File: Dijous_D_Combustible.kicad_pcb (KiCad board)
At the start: 2 copper layers, 90 x 75 mm, 64 parts, among them J1 Screw_Terminal_01x02, J2 Conn_01x02, J3 Conn_02x03_Counter_Clockwise, J4 DE9_Plug, J5 Conn_01x02, J6 Conn_01x02, J7 Conn_01x02, K1 Fujitsu_FTR-LYAA005x, K2 Fujitsu_FTR-LYAA005x, Q1 2SC4213, Q2 2SC4213, SW1 SW_Push, U1 MCP2551-I-SN, U2 LM2596S-ADJ, U3 PIC18F258-I/SO, U4 LM1117DT-5.0, U5 MCP4725xxx-xCH, Y1 HC-49-US

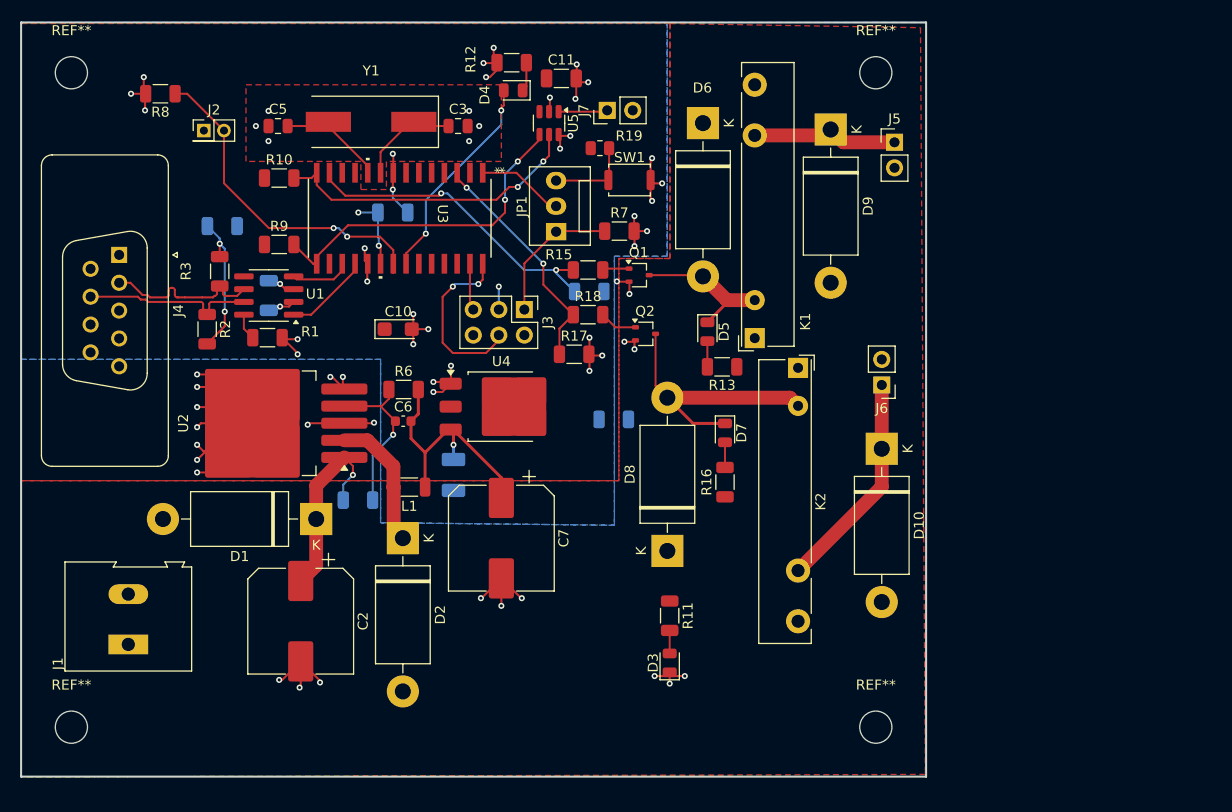
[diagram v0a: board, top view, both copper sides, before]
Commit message: Layout & README
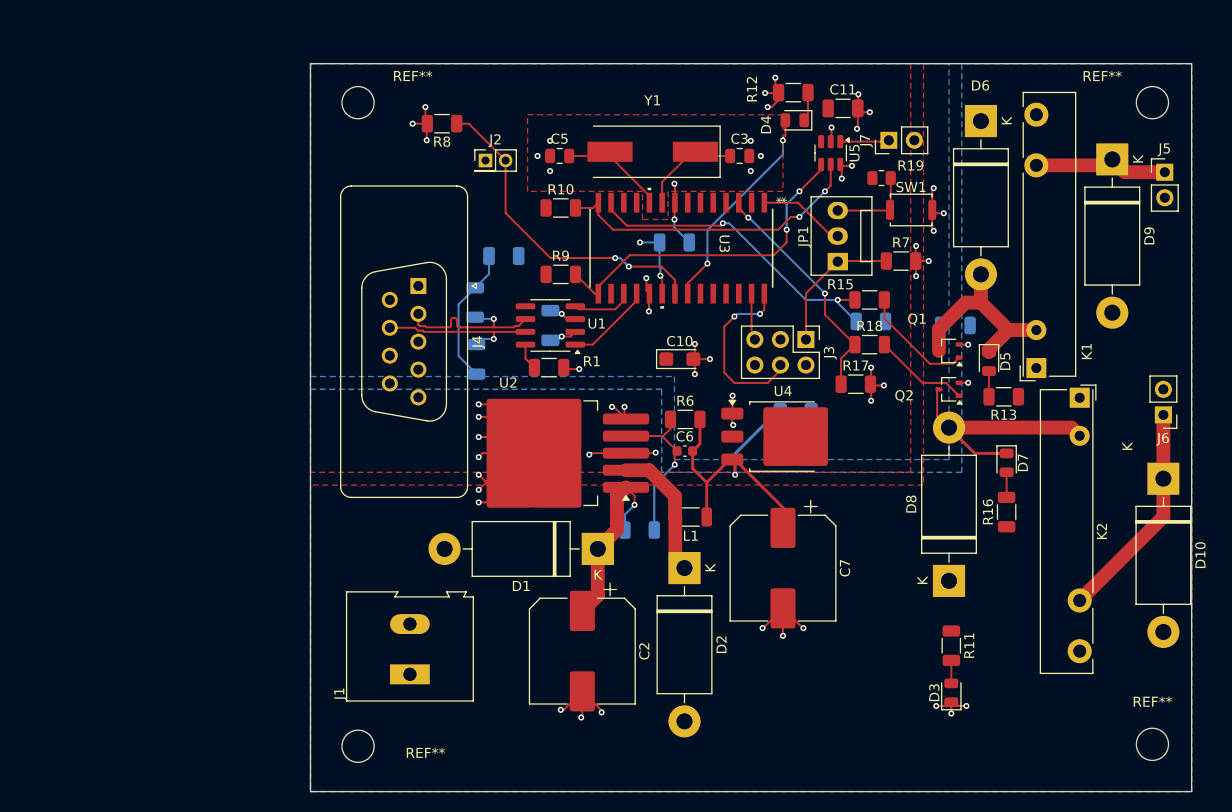
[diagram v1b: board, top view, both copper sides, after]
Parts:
- removed the REF** at (184.5, 137.1)
- removed the REF** at (104.5, 137.1)
- removed the REF** at (104.5, 72.0)
- removed the REF** at (184.5, 72.0)
- added REF**: MountingHole_3.2mm_M3, MountingHole:MountingHole_3.2mm_M3, F.Cu at (133.0, 75.0)
- added REF**: MountingHole_3.2mm_M3, MountingHole:MountingHole_3.2mm_M3, F.Cu at (133.0, 139.0)
- added REF**: MountingHole_3.2mm_M3, MountingHole:MountingHole_3.2mm_M3, F.Cu at (212.0, 138.8)
- added REF**: MountingHole_3.2mm_M3, MountingHole:MountingHole_3.2mm_M3, F.Cu at (212.0, 75.0)
- R2, R3: moved to B.Cu
- moved R4 35.2 mm to (192.4, 97.2)
- moved C8 34.6 mm to (176.5, 106.0), turned to 0 degrees
- moved Q1 31.7 mm to (191.8, 99.7), turned to 180 degrees
- moved Q2 30.7 mm to (191.8, 103.5), turned to 180 degrees
- moved J4 29.9 mm to (139.0, 93.2)
- moved C10 28.2 mm to (165.0, 100.5)
- moved C11 28.2 mm to (181.2, 75.6)
- moved C3 28.2 mm to (171.0, 80.3)
- moved C5 28.2 mm to (153.1, 80.3)
- moved C6 28.2 mm to (165.5, 109.7)
- moved C9 28.2 mm to (164.5, 88.9)
- moved D3 28.2 mm to (192.0, 133.7)
- moved D4 28.2 mm to (176.4, 76.8)
- moved D5 28.2 mm to (195.8, 100.8)
- moved D7 28.2 mm to (197.5, 110.8)
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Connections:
- C1 pad 1: (no net) -> +5V
- C1 pad 2: (no net) -> GND
- C10 pad 1: (no net) -> +5V
- C10 pad 2: (no net) -> GND
- C11 pad 1: (no net) -> +5V
- C11 pad 2: (no net) -> GND
- C2 pad 1: (no net) -> Vin_Buck
- C2 pad 2: (no net) -> GNDPWR
- C3 pad 1: (no net) -> /OSC1
- C3 pad 2: (no net) -> GND
- C4 pad 1: (no net) -> Net-(C4-Pad1)
- C4 pad 2: (no net) -> GND
- C5 pad 1: (no net) -> GND
- C5 pad 2: (no net) -> /OSC2
- C6 pad 1: (no net) -> Net-(U2-FB)
- C6 pad 2: (no net) -> Vin_LDO
- C7 pad 1: (no net) -> Vin_LDO
- C7 pad 2: (no net) -> GNDPWR
- C8 pad 1: (no net) -> Vin_LDO
- C8 pad 2: (no net) -> GND
- C9 pad 1: (no net) -> GND
- C9 pad 2: (no net) -> +5V
- D1 pad 1: (no net) -> Vin_Buck
- D1 pad 2: (no net) -> Vbat
- D10 pad 1: (no net) -> Solenoide
- D10 pad 2: (no net) -> GNDPWR
- D2 pad 1: (no net) -> Vout_Buck
- D2 pad 2: (no net) -> GNDPWR
- D3 pad 1: (no net) -> GNDPWR
- D3 pad 2: (no net) -> Net-(D3-A)
- D4 pad 1: (no net) -> Net-(D4-K)
- D4 pad 2: (no net) -> LED_pneumatics
- D5 pad 1: (no net) -> Retorn_sol
- D5 pad 2: (no net) -> Net-(D5-A)
- D6 pad 1: (no net) -> Vbat
- D6 pad 2: (no net) -> Retorn_sol
- D7 pad 1: (no net) -> Retorn_dip
- D7 pad 2: (no net) -> Net-(D7-A)
- D8 pad 1: (no net) -> Vbat
- D8 pad 2: (no net) -> Retorn_dip
- D9 pad 1: (no net) -> Bomba_combustible
- D9 pad 2: (no net) -> GNDPWR
- J1 pad 1: (no net) -> GNDPWR
- J1 pad 2: (no net) -> Vbat
- J2 pad 1: (no net) -> GND
- J2 pad 2: (no net) -> Boto
- J3 pad 1: (no net) -> MCLR
- J3 pad 2: (no net) -> +5V
- J3 pad 3: (no net) -> GND
- J3 pad 4: (no net) -> PGD
- J3 pad 5: (no net) -> PGC
- J3 pad 6: (no net) -> unconnected-(J3-Pin_6-Pad6)
- J4 pad 1: (no net) -> unconnected-(J4-Pad1)
- J4 pad 2: (no net) -> /Can-
- J4 pad 3: (no net) -> unconnected-(J4-Pad3)
- J4 pad 4: (no net) -> unconnected-(J4-Pad4)
- J4 pad 5: (no net) -> unconnected-(J4-Pad5)
- J4 pad 6: (no net) -> unconnected-(J4-Pad6)
- J4 pad 7: (no net) -> /Can+
- J4 pad 8: (no net) -> unconnected-(J4-Pad8)
- J4 pad 9: (no net) -> unconnected-(J4-Pad9)
- J5 pad 1: (no net) -> Bomba_combustible
- J5 pad 2: (no net) -> GNDPWR
- J6 pad 1: (no net) -> Solenoide
- J6 pad 2: (no net) -> GNDPWR
- J7 pad 1: (no net) -> Nivell_combustible
- J7 pad 2: (no net) -> GND
- JP1 pad 1: (no net) -> MCLR
- JP1 pad 2: (no net) -> Net-(JP1-C)
- JP1 pad 3: (no net) -> Net-(JP1-B)
- K1 pad 13: (no net) -> Bomba_combustible
- K1 pad 14: (no net) -> Vbat
- K1 pad A1: (no net) -> Vbat
- K1 pad A2: (no net) -> Retorn_sol
- K2 pad 13: (no net) -> Solenoide
- K2 pad 14: (no net) -> Vbat
- K2 pad A1: (no net) -> Vbat
- K2 pad A2: (no net) -> Retorn_dip
- L1 pad 1: (no net) -> Vin_LDO
- L1 pad 2: (no net) -> Vout_Buck
- Q1 pad 1: (no net) -> Net-(Q1-B)
- Q1 pad 2: (no net) -> GNDPWR
- Q1 pad 3: (no net) -> Retorn_sol
- Q2 pad 1: (no net) -> Net-(Q2-B)
- Q2 pad 2: (no net) -> GNDPWR
- Q2 pad 3: (no net) -> Retorn_dip
- R1 pad 1: (no net) -> Net-(U1-Rs)
- R1 pad 2: (no net) -> GND
- R10 pad 1: (no net) -> +5V
- R10 pad 2: (no net) -> SCL
- R11 pad 1: (no net) -> Vbat
- R11 pad 2: (no net) -> Net-(D3-A)
- R12 pad 1: (no net) -> Net-(D4-K)
- R12 pad 2: (no net) -> GND
- R13 pad 1: (no net) -> Vbat
- R13 pad 2: (no net) -> Net-(D5-A)
- R14 pad 1: (no net) -> R_Bomba
- R14 pad 2: (no net) -> GND
- R15 pad 1: (no net) -> R_Bomba
- R15 pad 2: (no net) -> Net-(Q1-B)
- R16 pad 1: (no net) -> Vbat
- R16 pad 2: (no net) -> Net-(D7-A)
- R17 pad 1: (no net) -> R_Dipòsit
- R17 pad 2: (no net) -> GND
- R18 pad 1: (no net) -> R_Dipòsit
- R18 pad 2: (no net) -> Net-(Q2-B)
- R19 pad 1: (no net) -> +5V
- R19 pad 2: (no net) -> Net-(JP1-B)
- R2 pad 1: (no net) -> /Can+
- R2 pad 2: (no net) -> Net-(C4-Pad1)
- R3 pad 1: (no net) -> Net-(C4-Pad1)
- R3 pad 2: (no net) -> /Can-
- R4 pad 1: (no net) -> GNDPWR
- R4 pad 2: (no net) -> GND
- R5 pad 1: (no net) -> Net-(U2-FB)
- R5 pad 2: (no net) -> Vin_Buck
- R6 pad 1: (no net) -> Net-(U2-FB)
- R6 pad 2: (no net) -> Vin_LDO
- R7 pad 1: (no net) -> MCLR
- R7 pad 2: (no net) -> GND
- R8 pad 1: (no net) -> Boto
- R8 pad 2: (no net) -> GND
- R9 pad 1: (no net) -> +5V
- R9 pad 2: (no net) -> SCA
- SW1 pad 1: (no net) -> Net-(JP1-B)
- SW1 pad 2: (no net) -> GND
- U1 pad 1: (no net) -> TXD
- U1 pad 2: (no net) -> GND
- U1 pad 3: (no net) -> +5V
- U1 pad 4: (no net) -> RXD
- U1 pad 5: (no net) -> unconnected-(U1-Vref-Pad5)
- U1 pad 6: (no net) -> /Can-
- U1 pad 7: (no net) -> /Can+
- U1 pad 8: (no net) -> Net-(U1-Rs)
- U2 pad 1: (no net) -> Vin_Buck
- U2 pad 2: (no net) -> Vout_Buck
- U2 pad 3: (no net) -> GNDPWR
- U2 pad 4: (no net) -> Net-(U2-FB)
- U2 pad 5: (no net) -> GNDPWR
- U3 pad 1: (no net) -> Net-(JP1-C)
- U3 pad 10: (no net) -> /OSC2
- U3 pad 11: (no net) -> unconnected-(U3A-RC0/T1OSO/T1CK1-Pad11)
- U3 pad 12: (no net) -> unconnected-(U3A-RC1/T1OSI-Pad12)
- U3 pad 13: (no net) -> R_Bomba
- U3 pad 14: (no net) -> SCL
- U3 pad 15: (no net) -> SCA
- U3 pad 16: (no net) -> unconnected-(U3A-RC5/SDO-Pad16)
- U3 pad 17: (no net) -> RXD
- U3 pad 18: (no net) -> TXD
- U3 pad 19: (no net) -> GND
- U3 pad 2: (no net) -> unconnected-(U3A-RA0/AN0/CVREF-Pad2)
- U3 pad 20: (no net) -> +5V
- U3 pad 21: (no net) -> Boto
- U3 pad 22: (no net) -> LED_pneumatics
- U3 pad 23: (no net) -> unconnected-(U3A-RB2/CANTX/INT2-Pad23)
- U3 pad 24: (no net) -> unconnected-(U3A-RB3/CANRX-Pad24)
- U3 pad 25: (no net) -> unconnected-(U3A-RB4-Pad25)
- U3 pad 26: (no net) -> unconnected-(U3A-RB5/PGM-Pad26)
- U3 pad 27: (no net) -> PGC
- U3 pad 28: (no net) -> PGD
- U3 pad 3: (no net) -> R_Dipòsit
- U3 pad 4: (no net) -> unconnected-(U3A-RA2/AN2/VREF--Pad4)
- U3 pad 5: (no net) -> unconnected-(U3A-RA3/AN3/VREF+-Pad5)
- U3 pad 6: (no net) -> unconnected-(U3A-RA4/T0CKI-Pad6)
- U3 pad 7: (no net) -> unconnected-(U3A-RA5/AN4/*SS/LVDIN-Pad7)
- U3 pad 8: (no net) -> GND
- U3 pad 9: (no net) -> /OSC1
- U4 pad 1: (no net) -> GND
- U4 pad 2: (no net) -> +5V
- U4 pad 3: (no net) -> Vin_LDO
- U5 pad 1: (no net) -> Nivell_combustible
- U5 pad 2: (no net) -> GND
- U5 pad 3: (no net) -> +5V
- U5 pad 4: (no net) -> SCA
- U5 pad 5: (no net) -> SCL
- U5 pad 6: (no net) -> GND
- Y1 pad 1: (no net) -> /OSC1
- Y1 pad 2: (no net) -> /OSC2
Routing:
- net (no net): track 627.4 -> 0.00 mm, vias 87 -> 0
- net GNDPWR: track 0.00 -> 60.2 mm, vias 0 -> 22
- net GND: track 0.00 -> 56.0 mm, vias 0 -> 38
- net Boto: track 0.00 -> 34.1 mm, vias 0 -> 2
- net SCA: track 0.00 -> 33.5 mm, vias 0 -> 2
- net Vin_LDO: track 0.00 -> 32.7 mm, vias 0 -> 1
- net R_Bomba: track 0.00 -> 31.8 mm, vias 0 -> 2
- net SCL: track 0.00 -> 31.3 mm, vias 0 -> 2
- net Retorn_dip: track 0.00 -> 24.5 mm
- net R_Dipòsit: track 0.00 -> 23.5 mm, vias 0 -> 2
- net Solenoide: track 0.00 -> 21.9 mm
- net LED_pneumatics: track 0.00 -> 21.3 mm, vias 0 -> 2
- net Retorn_sol: track 0.00 -> 19.9 mm
- net Vin_Buck: track 0.00 -> 19.1 mm, vias 0 -> 1
- net PGD: track 0.00 -> 17.9 mm, vias 0 -> 2
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- added copper zone on F.Cu, net +5V
- added copper zone on B.Cu, net GND
- added copper zone on F.Cu, net GND
- added copper zone on B.Cu, net GNDPWR
- added copper zone on F.Cu, net Vbat
- removed copper zone on B.Cu, net (none)
- removed copper zone on F.Cu, net (none)
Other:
- board size 90 x 75 mm -> 87.6 x 72.4 mm
